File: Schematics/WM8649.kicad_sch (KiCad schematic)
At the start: 6 parts, among them J10 Line In, J11 BOB21250-LEFT, J12 BOB21250-RIGHT, J9 Line In

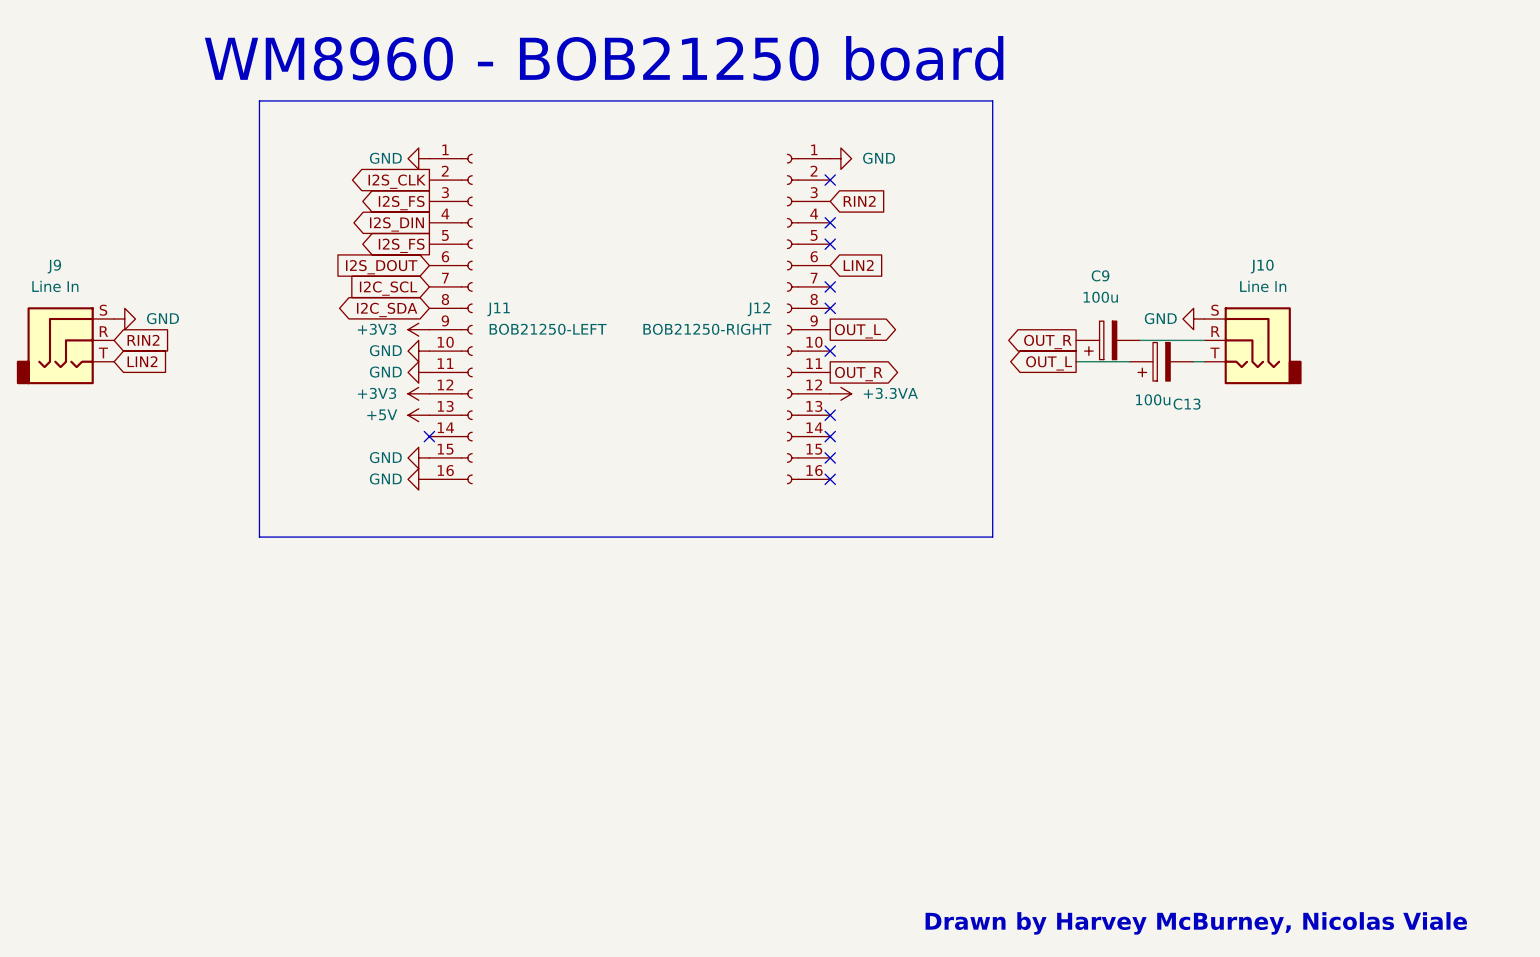
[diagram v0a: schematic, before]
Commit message: Tidied up Schematic
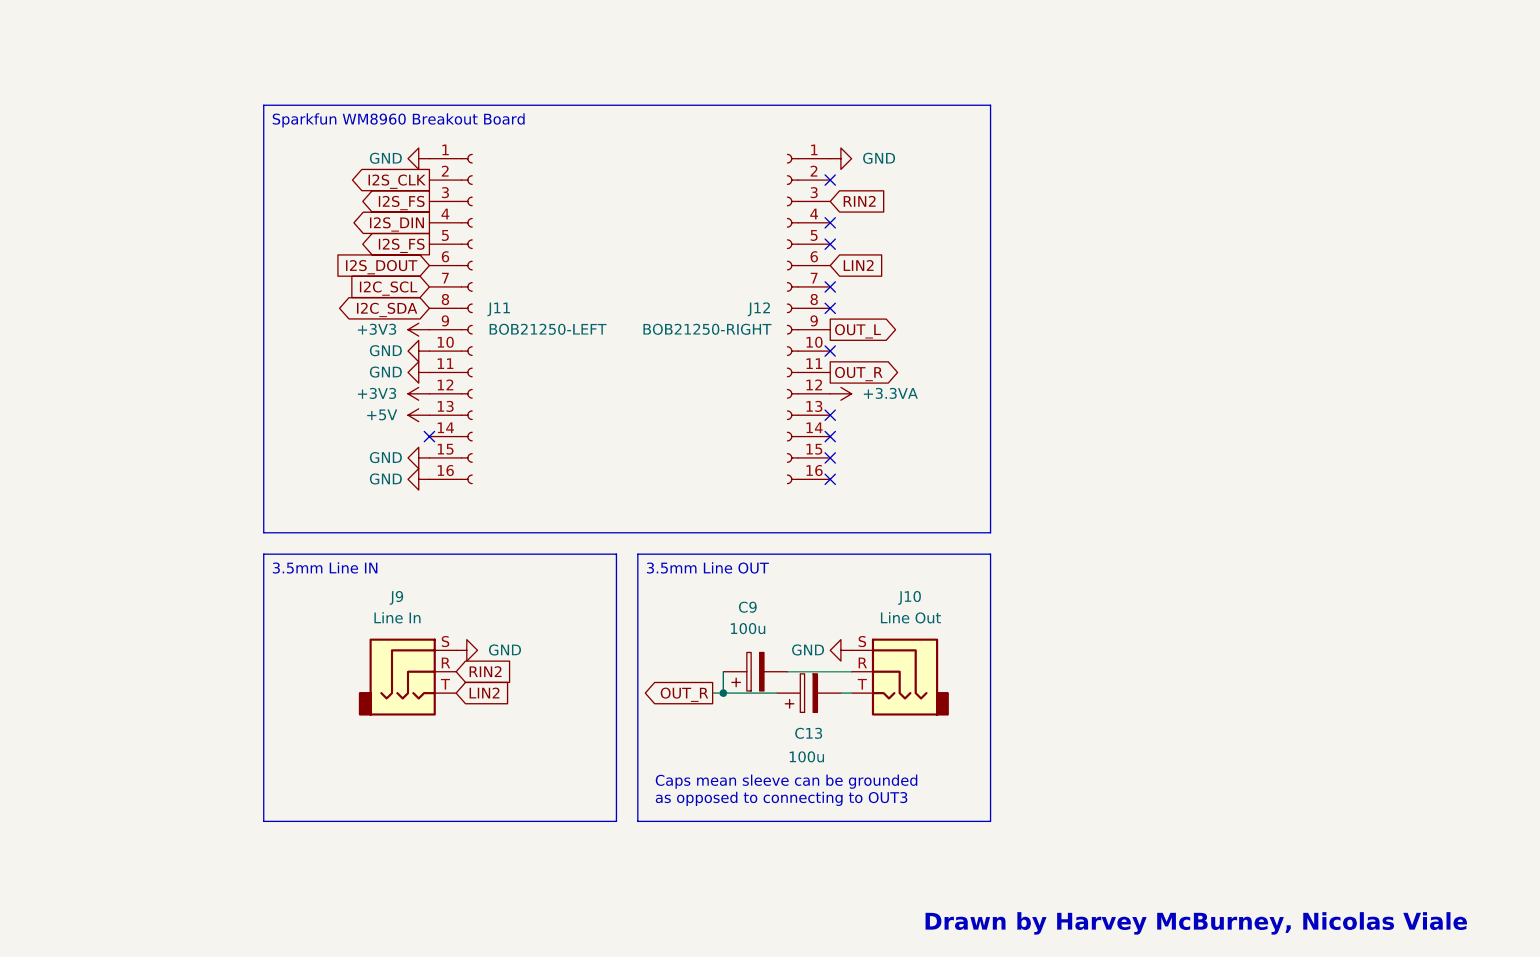
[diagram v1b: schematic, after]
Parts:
- J10: value Line In -> Line Out
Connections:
- net OUT_L: no longer C13.1
- net OUT_R: now also C13.1
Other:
- note added: "Caps mean sleeve can be grounded as opposed to connecting to OUT3"
- note removed: "WM8960 - BOB21250 board"
- moved on the sheet: C13, C9, J10, J9
